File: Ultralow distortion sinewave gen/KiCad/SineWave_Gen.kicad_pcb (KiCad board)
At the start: 4 copper layers, 100 x 90 mm, 74 parts, among them J10 Jumper, J2 SINE_OUT, J8 Jumper, P1 Conn_01x05, Q1 MMBT3904, U1 LT1468, U16 LT3045xMSE, U17 LT3094xMSE, U2 LT1468, U3 LT1468, U4 NSL-32, U5 LT1122, U6 LT1122, U7 LT1122, U8 LT1006, U9 LT1634-5

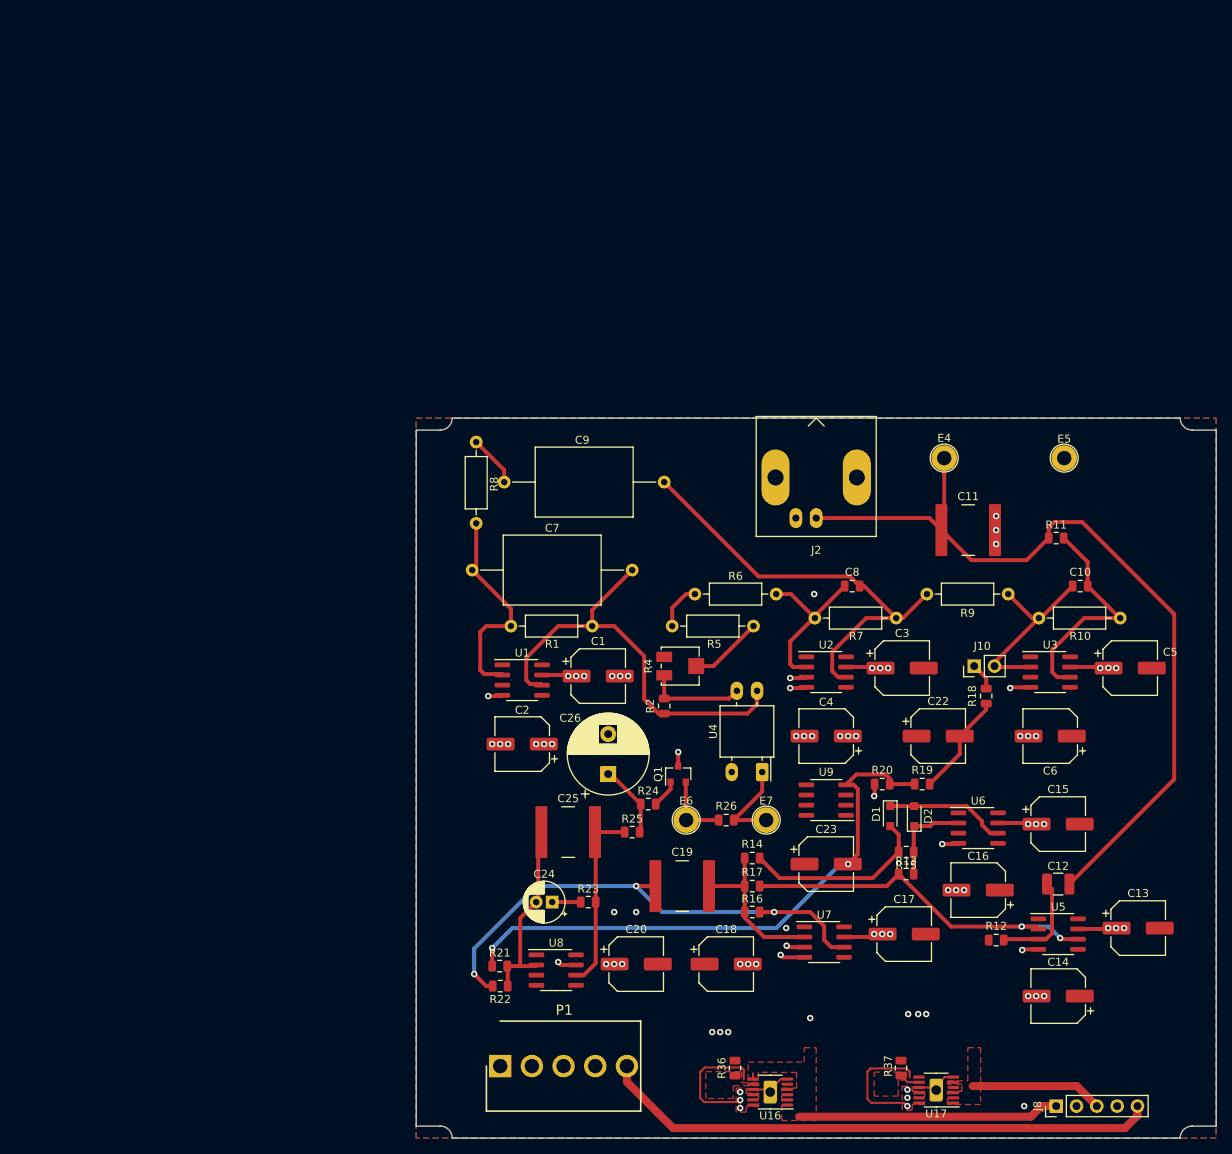
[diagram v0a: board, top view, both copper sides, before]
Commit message: update
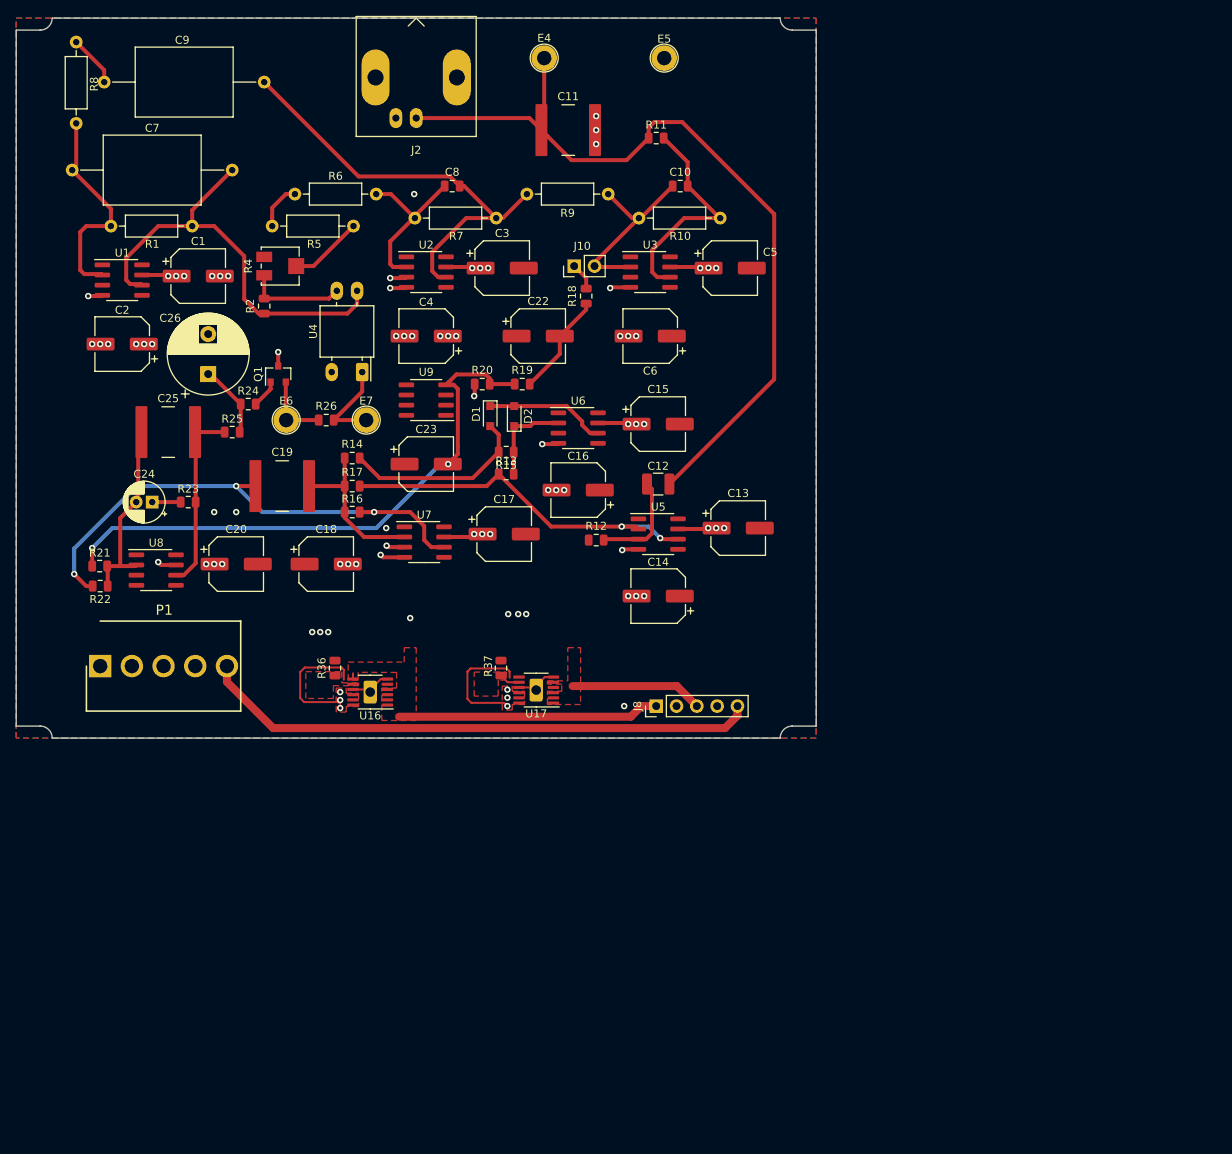
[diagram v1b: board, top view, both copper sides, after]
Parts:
- moved C1 70.7 mm to (-27.2, -17.8)
- moved C10 70.7 mm to (33.0, -29.0)
- moved C11 70.7 mm to (19.0, -36.0)
- moved C12 70.7 mm to (30.2, 8.25)
- moved C13 70.7 mm to (40.2, 13.8)
- moved C14 70.7 mm to (30.2, 22.2)
- moved C15 70.7 mm to (30.2, 0.75)
- moved C16 70.7 mm to (20.2, 9.00)
- moved C17 70.7 mm to (11.0, 14.5)
- moved C18 70.7 mm to (-11.2, 18.2)
- moved C19 70.7 mm to (-16.8, 8.50)
- moved C2 70.7 mm to (-36.8, -9.25)
- moved C20 70.7 mm to (-22.5, 18.2)
- moved C22 70.7 mm to (15.2, -10.2)
- moved C23 70.7 mm to (1.25, 5.75)
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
